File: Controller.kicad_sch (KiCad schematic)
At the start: 37 parts, among them IC3 STM32H563VGT6, U5 TCAN1042VDRBRQ1

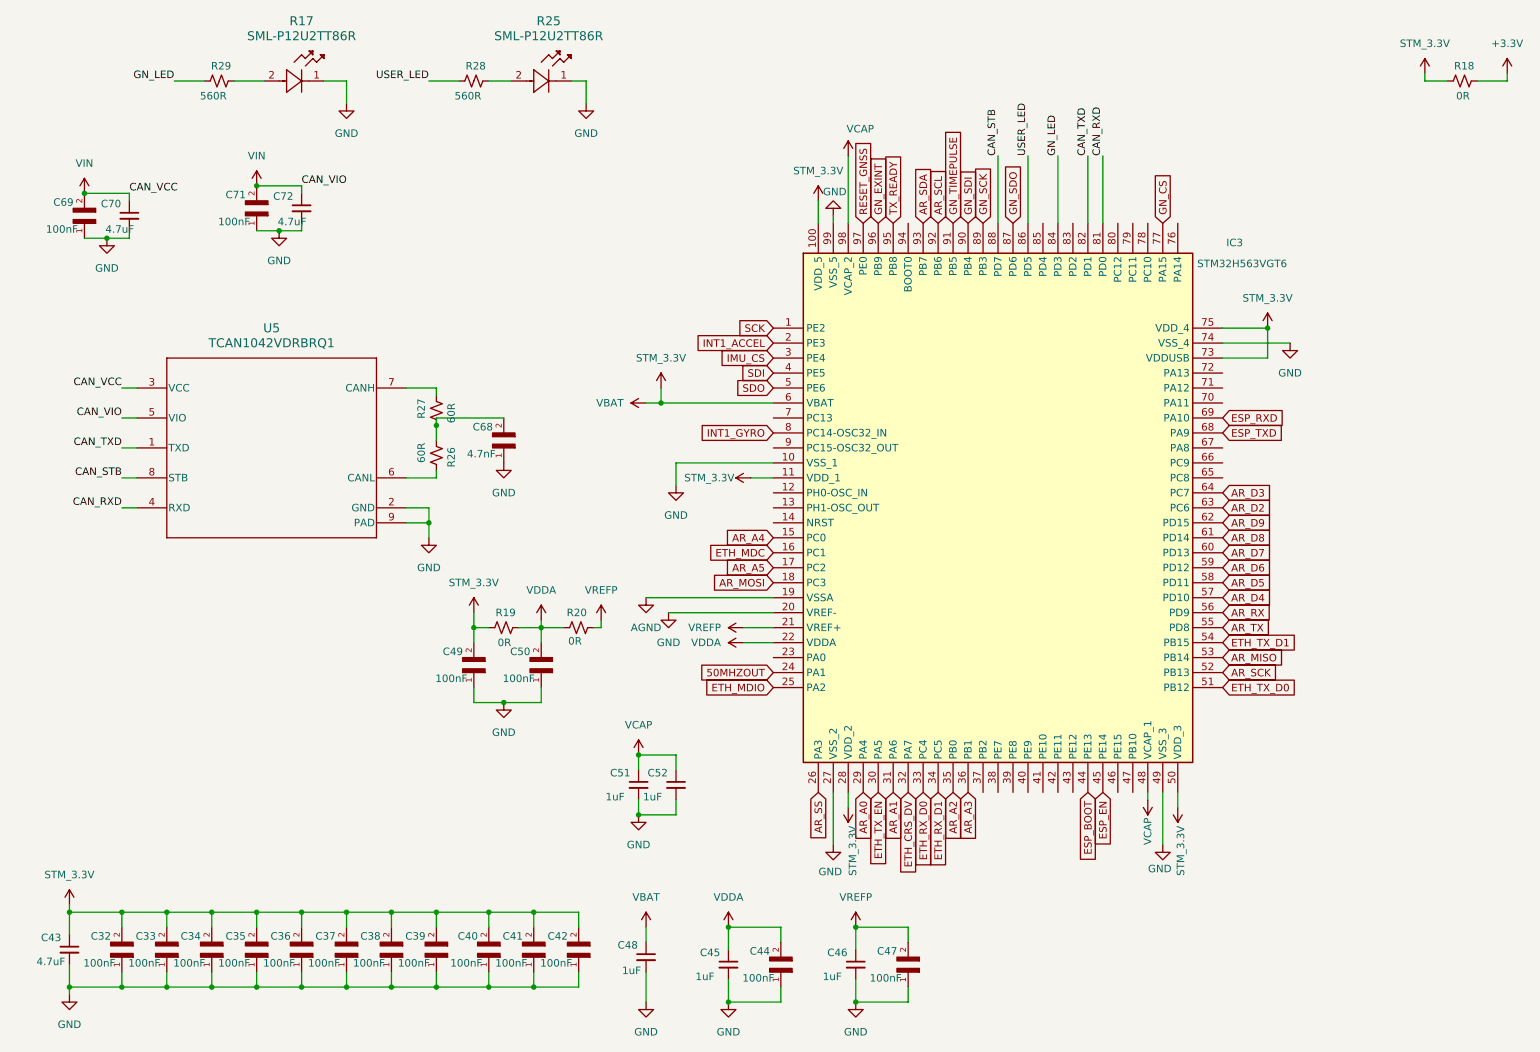
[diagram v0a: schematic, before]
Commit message: new
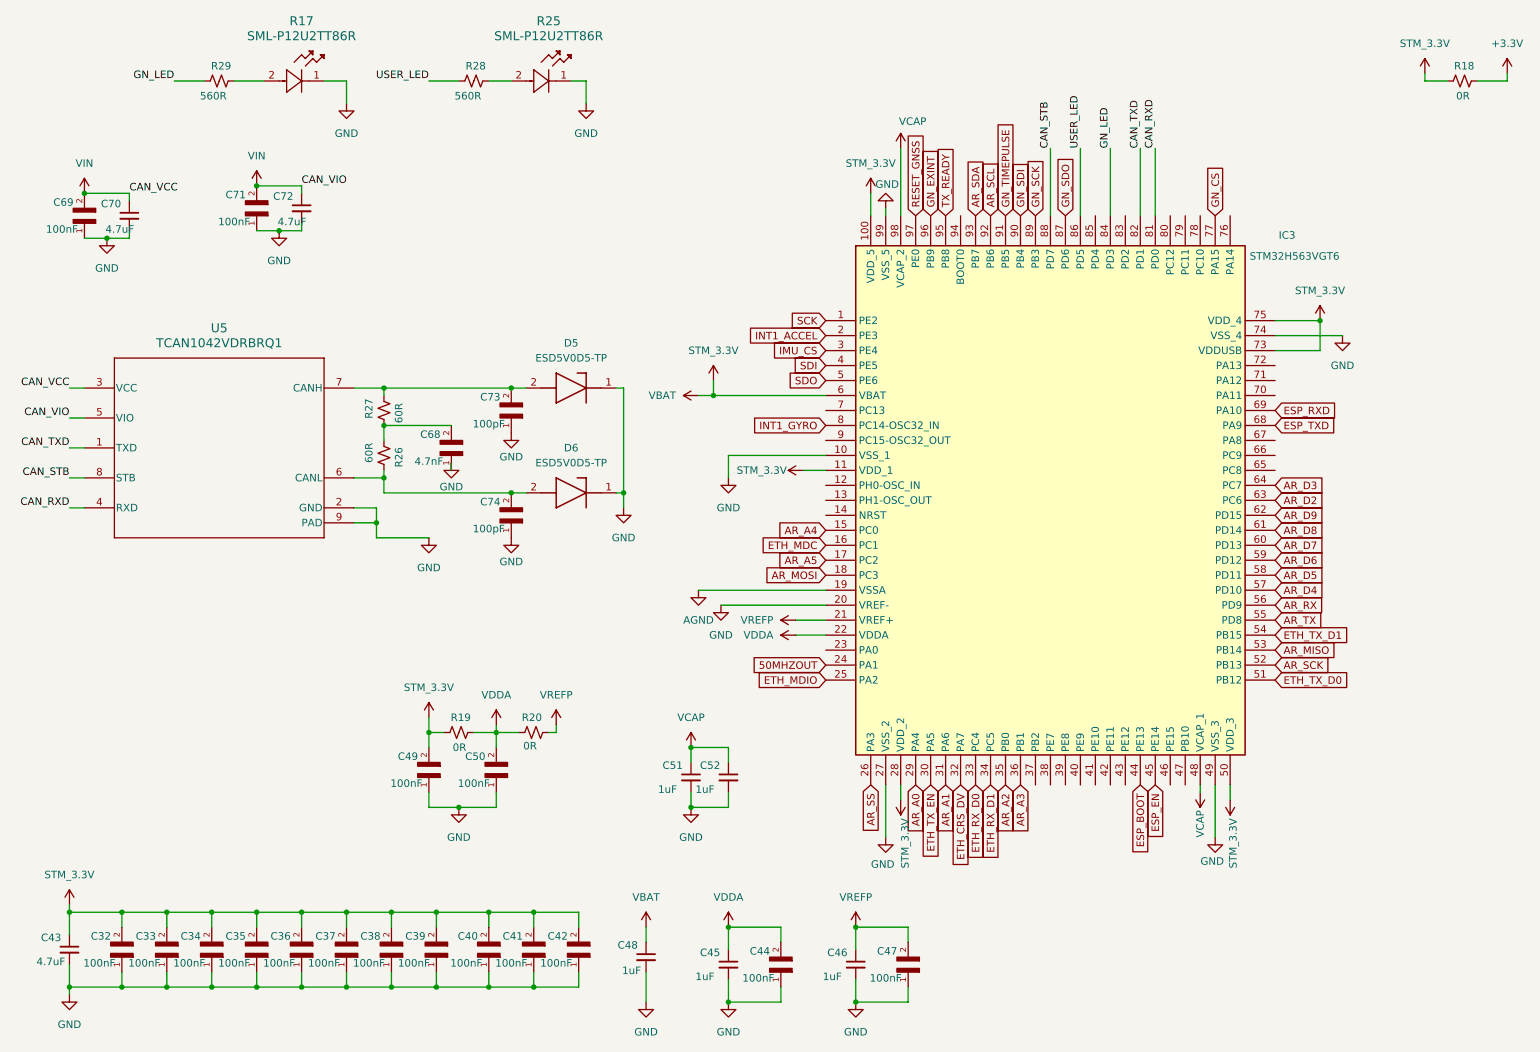
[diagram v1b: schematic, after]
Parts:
- added C73, C74: 100pF, C0402C104K4RAC:CAPC1005X55N, symbol C0402C104K4RAC:C0402C104K4RAC
- added D5, D6: ESD5V0D5-TP, ESD5V0D5TP, symbol ESD5V0D5-TP:ESD5V0D5-TP
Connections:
- net GND: now also C73.1, C74.1, D5.1 (K), D6.1 (K)
- net at R26.2, U5.6 (CANL): now also C74.2, D6.2 (A)
- net at R27.2, U5.7 (CANH): now also C73.2, D5.2 (A)
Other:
- moved on the sheet: C49, C50, C51, C52, C68, IC3, R19, R20, R26, R27, U5
